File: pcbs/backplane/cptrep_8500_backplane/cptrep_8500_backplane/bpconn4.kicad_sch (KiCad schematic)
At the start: 1 part, among them J4 cpt-backplane_100

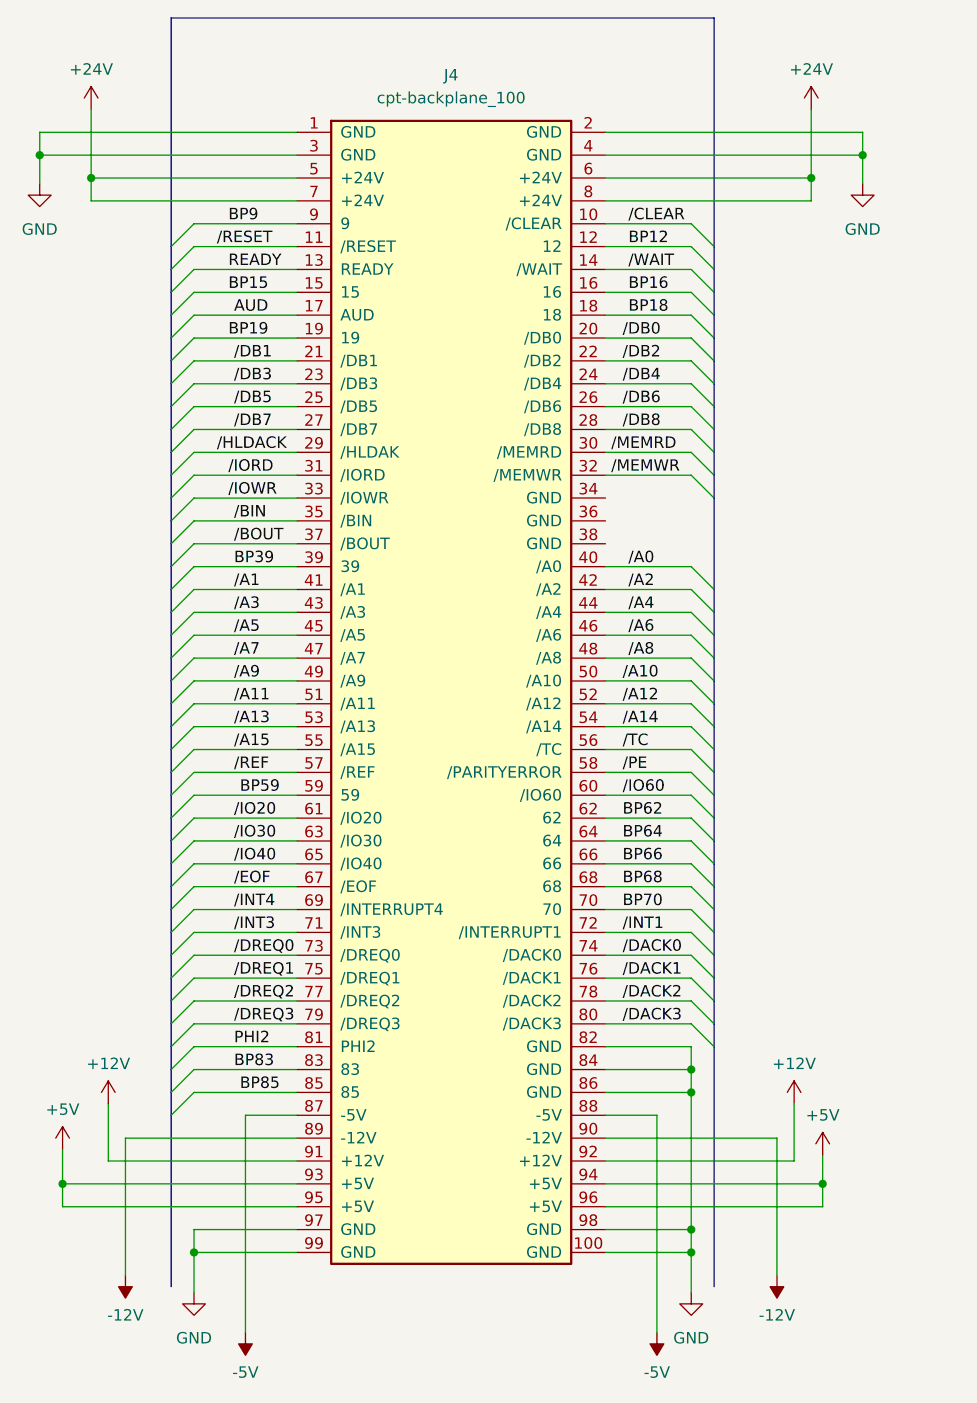
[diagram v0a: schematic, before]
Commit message: "Update"
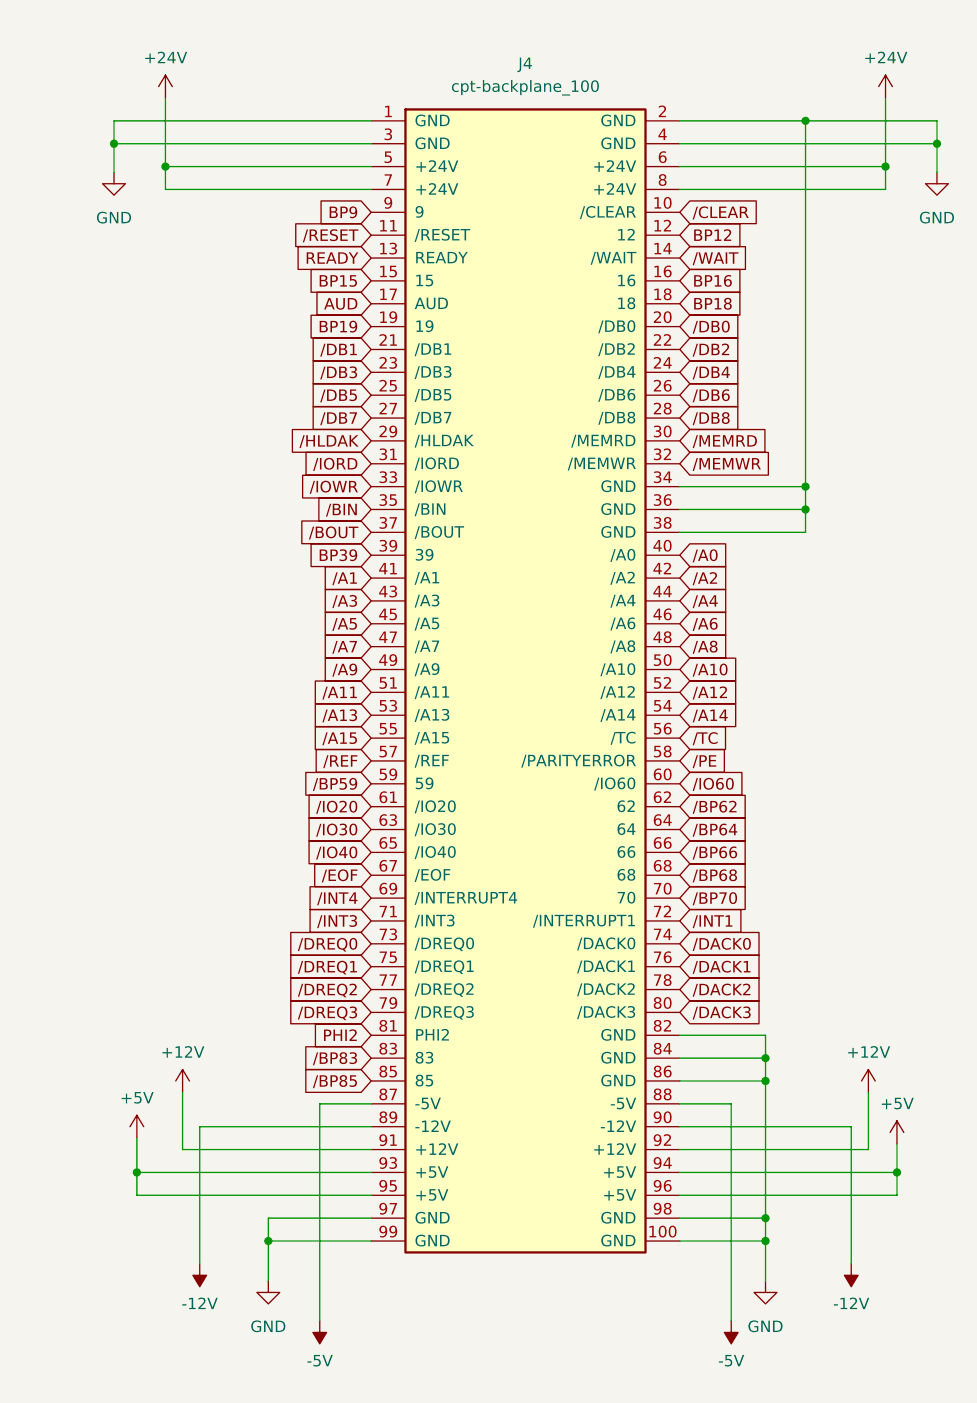
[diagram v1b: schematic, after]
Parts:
- J4: footprint (none) -> ajm-cpt:cpt-8500-backplane-connector
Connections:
- net GND: now also J4.34 (GND), J4.36 (GND), J4.38 (GND)
- net /BP68: now reaches J4.68
- net BP59 renamed /BP59
- net BP62 renamed /BP62
- net BP64 renamed /BP64
- net BP66 renamed /BP66
- net BP70 renamed /BP70
- net BP83 renamed /BP83
- net BP85 renamed /BP85
- net /HLDACK renamed /HLDAK
